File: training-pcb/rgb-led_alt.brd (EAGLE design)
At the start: 30 x 30 mm, 23 parts, among them J1 MICRO-USB, J2 AVR_SPI_PROG2PTH2, U1 ATTINY441/841SSU/SSUR, U2 PCA9533

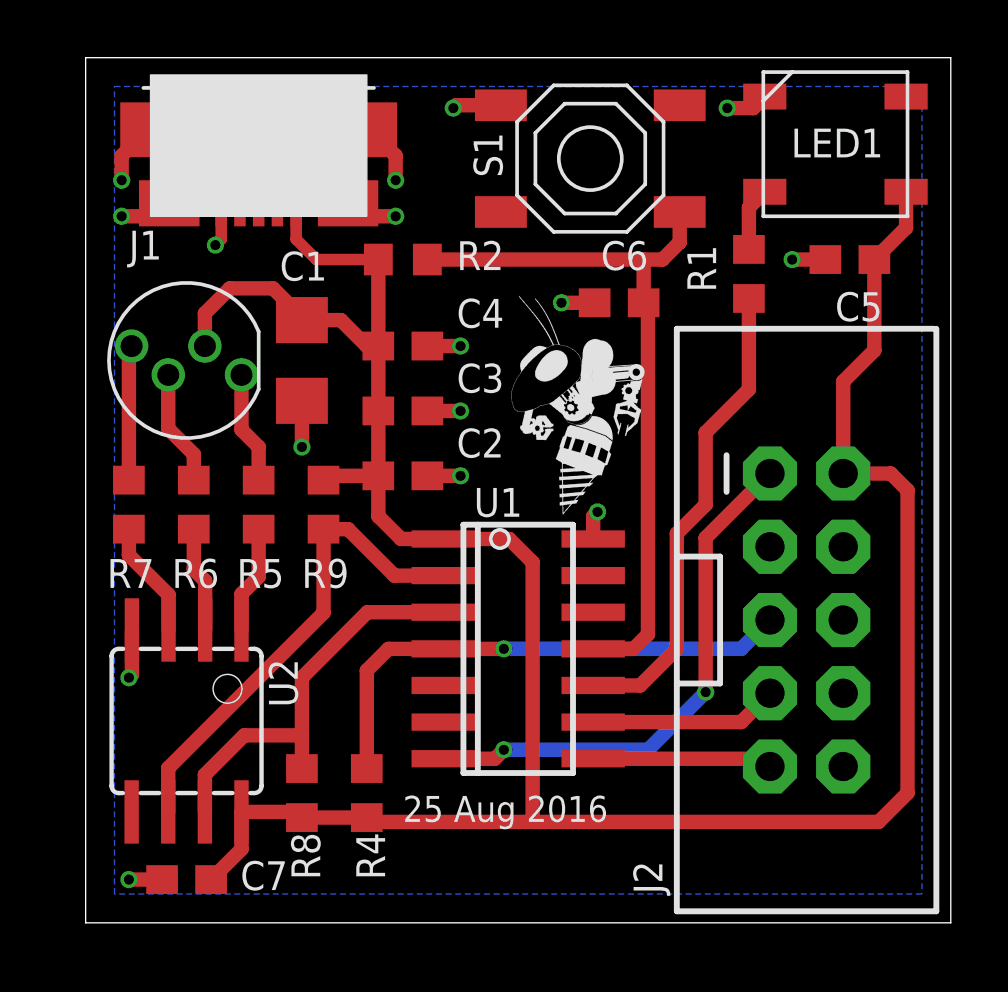
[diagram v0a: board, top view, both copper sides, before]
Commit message: cheaters
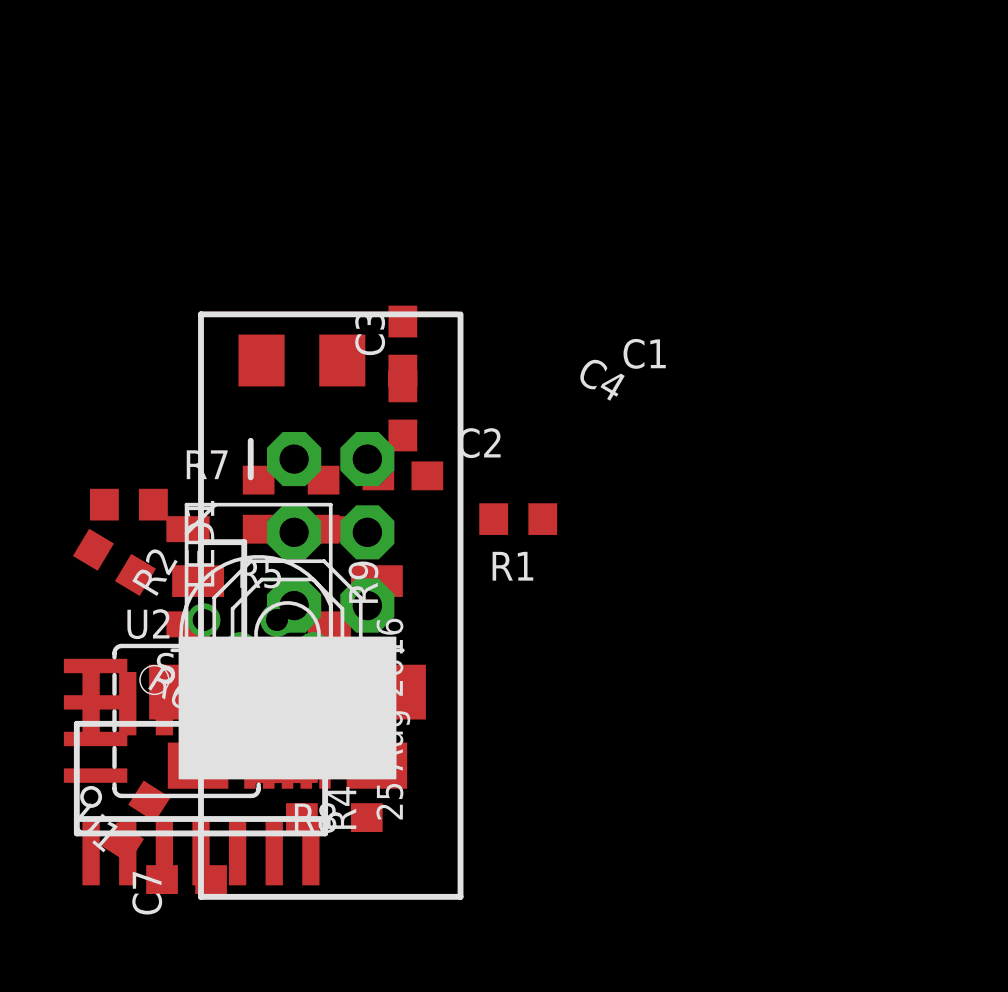
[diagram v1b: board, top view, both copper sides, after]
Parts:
- removed U$2: (no value), RoboJackets-Aesthetics:ROBOBUZZ_0.4X
- moved LED1 25.0 mm to (6.00, 12.0)
- moved C5 24.7 mm to (6.50, 8.50), turned to 270 degrees
- moved S1 19.6 mm to (7.00, 10.0)
- moved J1 19.5 mm to (7.00, 8.00)
- moved C6 18.4 mm to (8.50, 6.00)
- moved J2 16.5 mm to (8.50, 11.0)
- moved R2 14.5 mm to (1.00, 12.5), turned to 149.1 degrees
- moved U1 11.9 mm to (4.00, 5.00), turned to 0 degrees
- moved R1 11.7 mm to (15.0, 14.0), turned to 0 degrees
- moved R6 11.2 mm to (1.75, 3.50), turned to 57.4 degrees
- moved D1 9.82 mm to (6.00, 10.0)
- turned C1 to 0 degrees
- turned C3 to 90 degrees
- turned C4 to 90 degrees
- turned C7 to 0 degrees
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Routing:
- net +5V: track 88.6 -> 0.00 mm
- net GND: track 31.4 -> 0.00 mm, vias 16 -> 0
- net !BTN: track 25.2 -> 0.00 mm
- net MOSI: track 18.6 -> 0.00 mm, vias 2 -> 0
- net !RESET: track 18.1 -> 0.00 mm, vias 1 -> 0
- net SCL: track 16.9 -> 0.00 mm
- net LED_CNTRL: track 16.6 -> 0.00 mm
- net SDA: track 14.2 -> 0.00 mm
- net SCK: track 6.54 -> 0.00 mm
- net MISO: track 6.24 -> 0.00 mm
- net N$10: track 4.69 -> 0.00 mm
- net N$13: track 4.07 -> 0.00 mm
- net N$9: track 4.02 -> 0.00 mm
- net N$6: track 3.90 -> 0.00 mm
- net N$11: track 3.74 -> 0.00 mm
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- removed copper zone on layer 16, net GND
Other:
- board outline removed
